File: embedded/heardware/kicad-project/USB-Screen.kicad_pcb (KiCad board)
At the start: 2 copper layers, 32 x 34 mm, 21 parts, among them J1 USB_B_Micro, J2 Conn_01x04, Q1 NPN, U1 ZJY154T-PG04, U2 CH551, U3 SC662

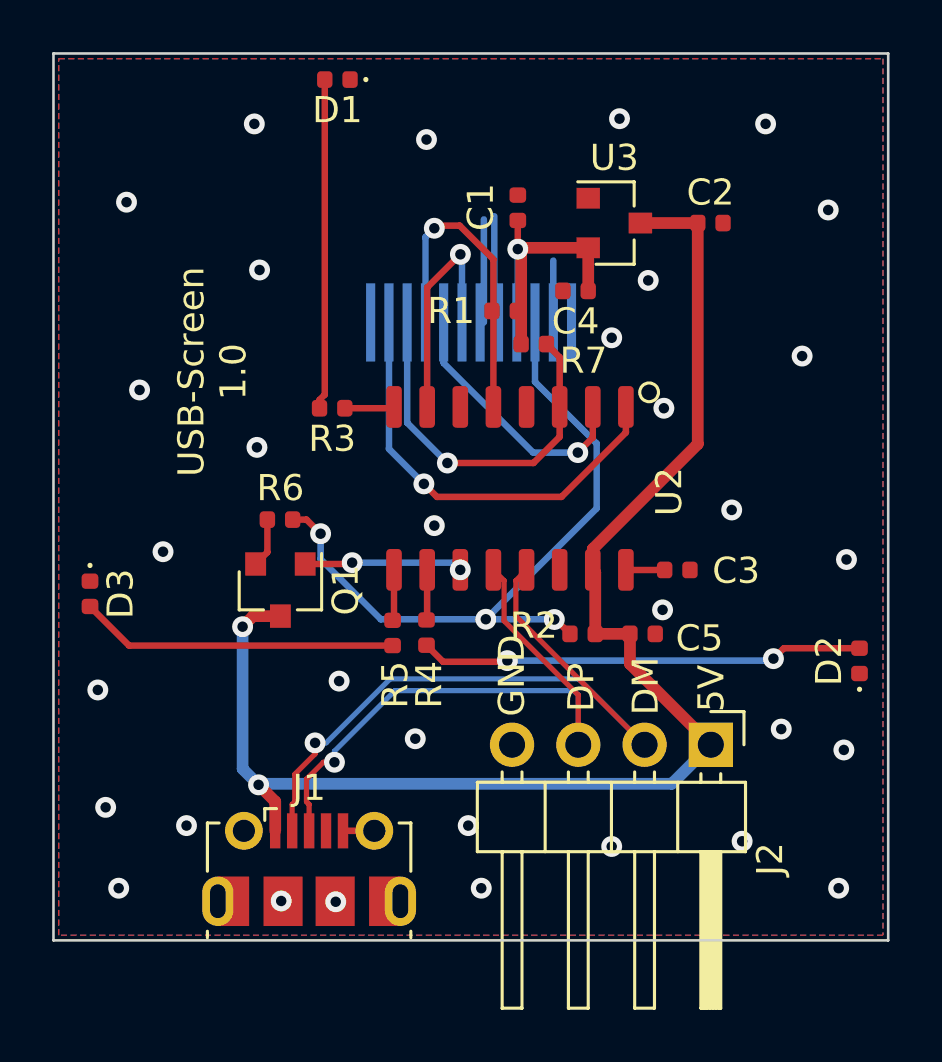
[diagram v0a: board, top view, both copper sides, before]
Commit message: 重新布线
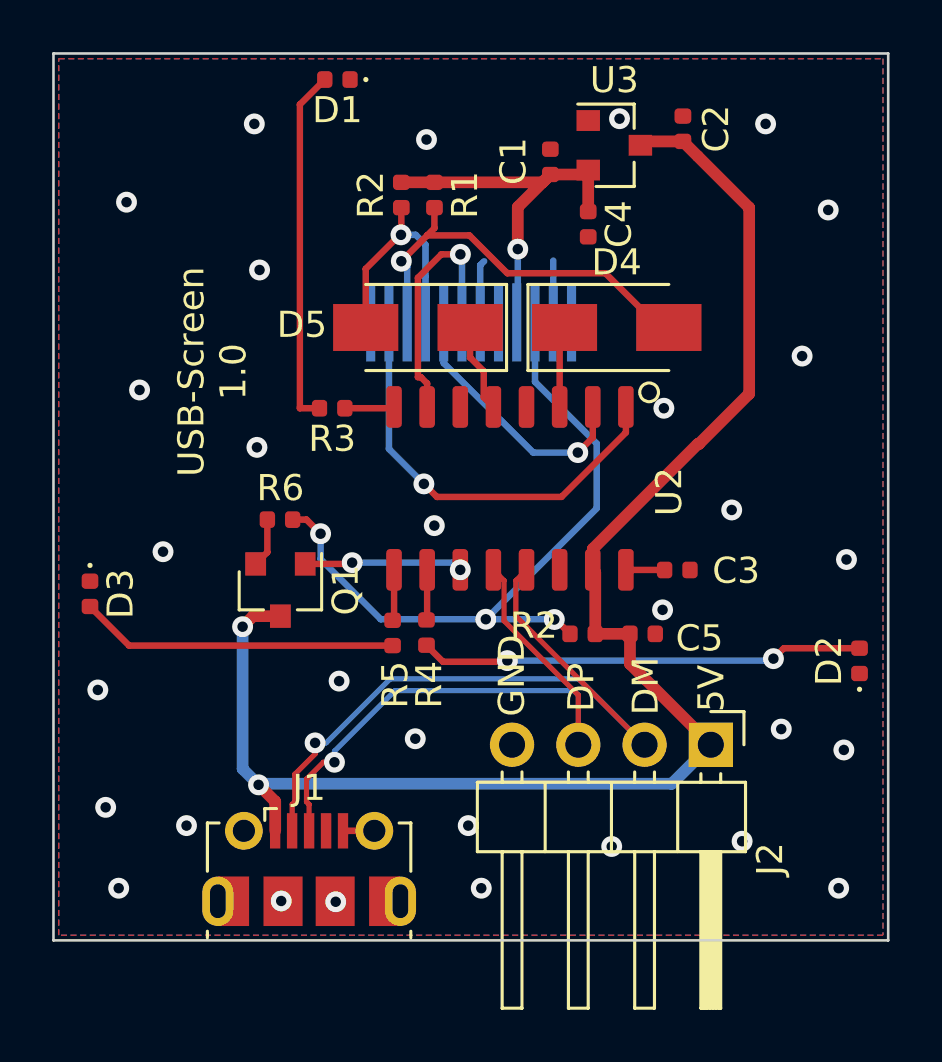
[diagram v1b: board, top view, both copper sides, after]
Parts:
- removed R7: 10K, Resistor_SMD:R_0402_1005Metric
- added D4: SS14, Diode_SMD:D_SMA, F.Cu at (118.6, 90.5)
- added D5: SS14, Diode_SMD:D_SMA, F.Cu at (111.0, 90.5)
- added R2: 10K, Resistor_SMD:R_0402_1005Metric, F.Cu at (110.3, 85.4)
- moved R1 5.20 mm to (111.6, 85.4), turned to 270 degrees
- moved C2 3.77 mm to (121.1, 82.9), turned to 90 degrees
- moved U3 2.98 mm to (118.5, 83.5)
- moved C4 2.60 mm to (117.5, 86.5), turned to 270 degrees
- moved C1 2.16 mm to (116.0, 84.2)
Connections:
- R1 pad 1: /SCL -> +3V3
- R1 pad 2: +3V3 -> /SDA
- U2 pad 3: /SDA -> Net-(D4-Pad1)
- U2 pad 5: /SCL -> Net-(D5-Pad1)
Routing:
- net GND: track 11.6 -> 6.68 mm, vias 33 -> 31
- net +5V: track 55.0 -> 59.5 mm
- net +3V3: track 12.0 -> 15.4 mm
- net Net-(D5-Pad1): track 0.00 -> 3.42 mm
- net Net-(D4-Pad1): track 0.00 -> 3.12 mm
- net /SCL: track 12.3 -> 9.27 mm
- net /SDA: track 14.5 -> 15.7 mm
- net Net-(D1-Pad2): track 12.7 -> 13.8 mm
- net /DC: track 9.01 -> 9.80 mm
